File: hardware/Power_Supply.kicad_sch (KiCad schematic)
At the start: 50 parts, among them IC1 LM13700, IC2 LM13700, IC3 LM13700, J1 USB_B, SW2 POWER, U2 TL064, U6 TL064

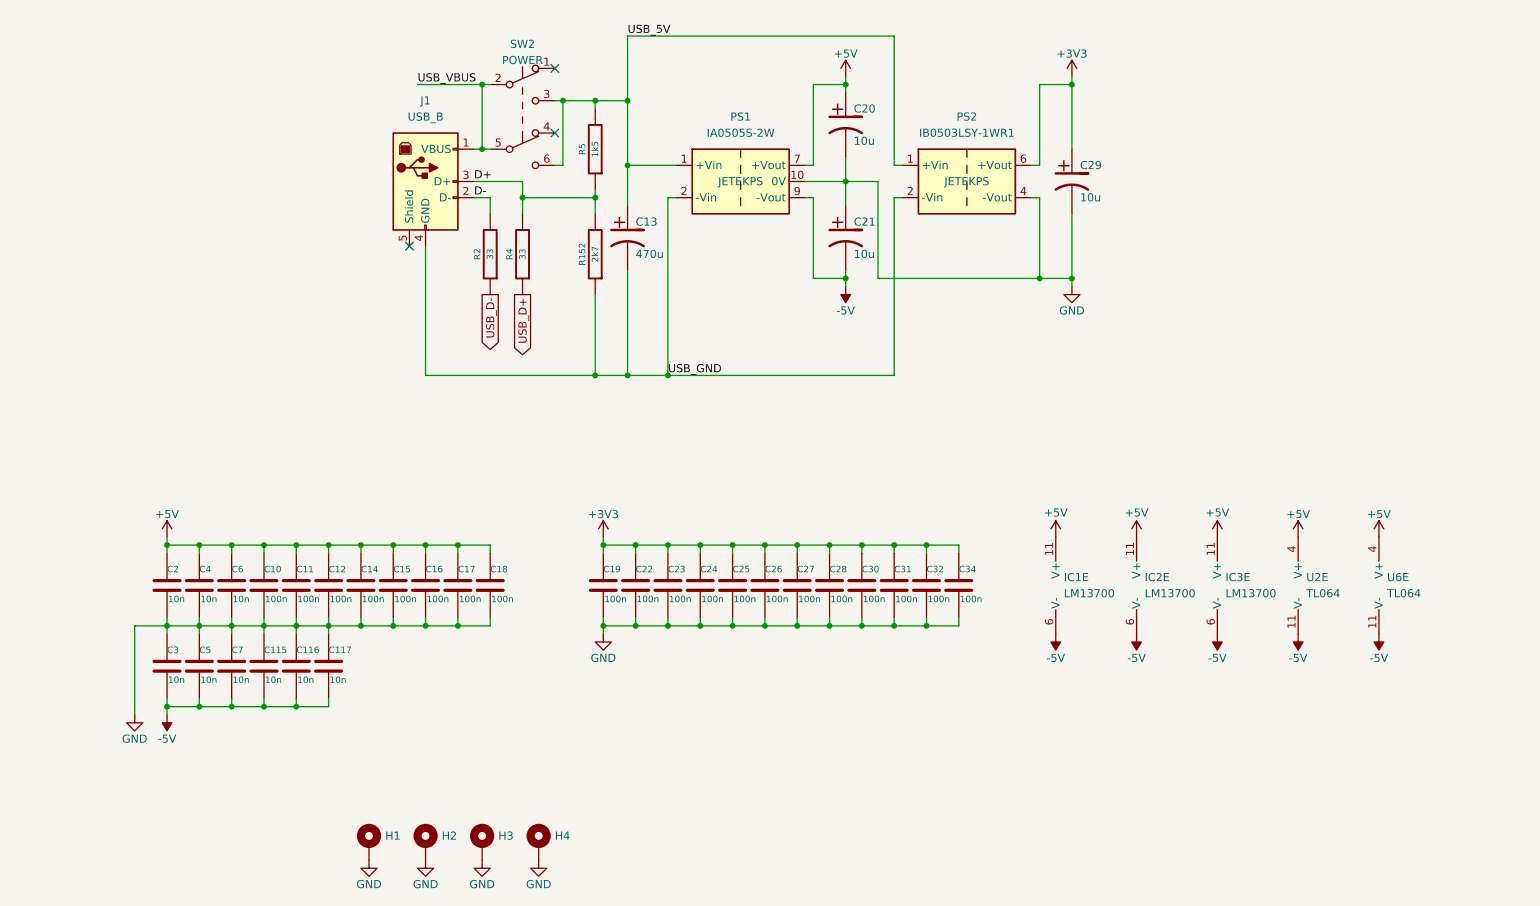
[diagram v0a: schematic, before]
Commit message: hardware: sch/pcb updates by Guimli
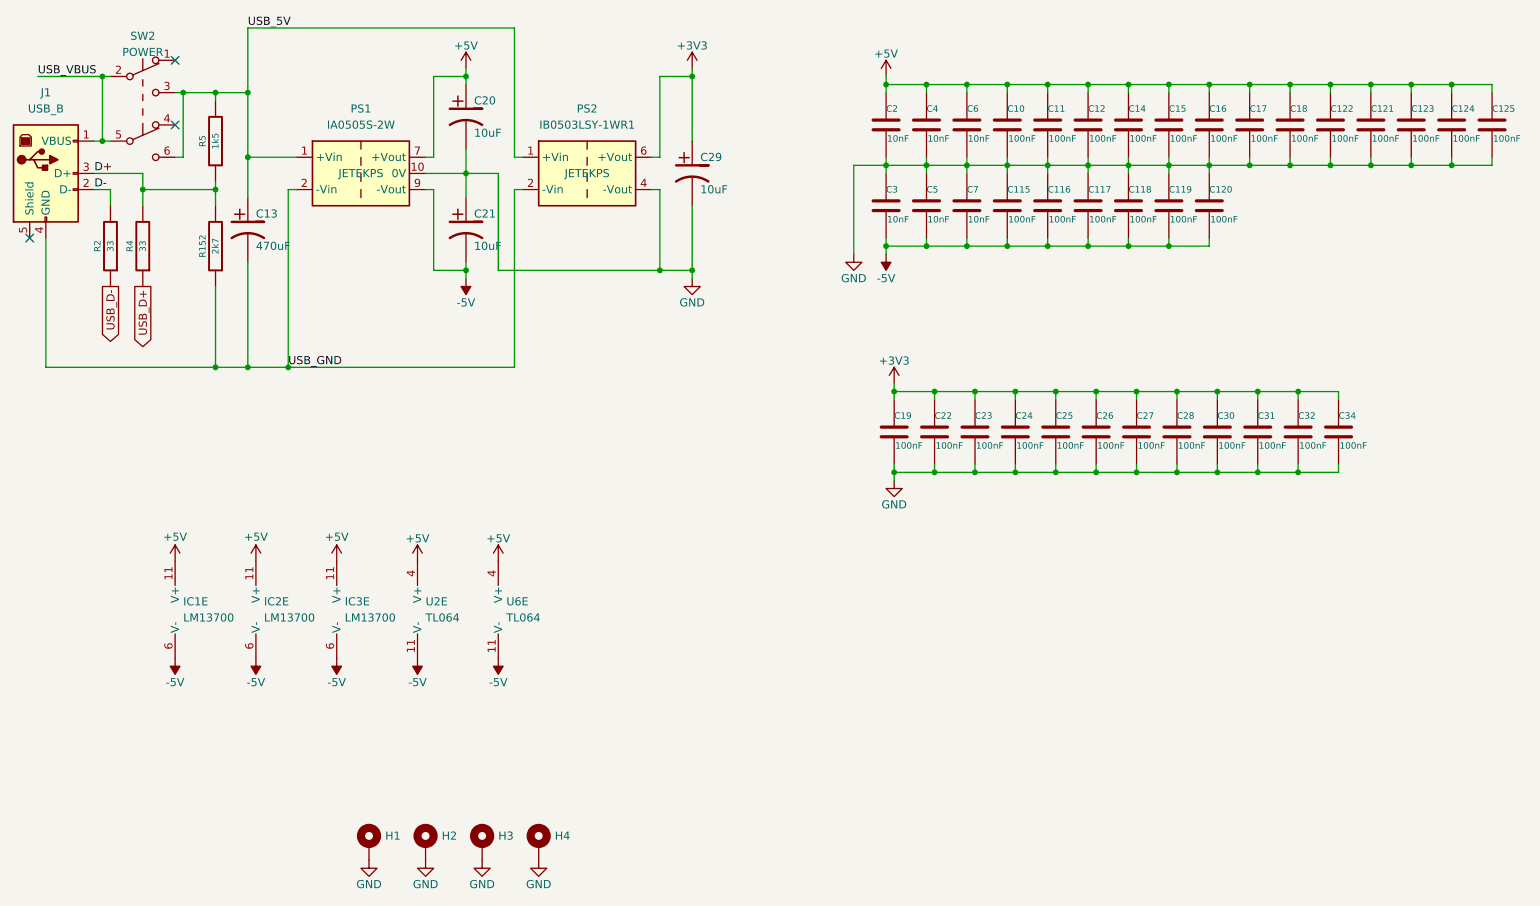
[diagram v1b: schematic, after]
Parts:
- added C118, C119, C120, C121, C122, C123, C124, C125: 100nF, Capacitor_SMD:C_0805_2012Metric, symbol Additional:C
- C10, C11, C12, C14, C15, C16, C17, C18, C19, C22, C23, C24, C25, C26, C27, C28, C30, C31, C32, C34: value 100n -> 100nF
- C115, C116, C117: value 10n -> 100nF; LCSC C1710 -> C28233
- C13: value 470u -> 470uF
- C2, C3, C4, C5, C6, C7: value 10n -> 10nF
- C20, C21, C29: value 10u -> 10uF
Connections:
- net +5V: now also C121.1, C122.1, C123.1, C124.1, C125.1
- net -5V: now also C118.2, C119.2, C120.2
- net GND: now also C118.1, C119.1, C120.1, C121.2, C122.2, C123.2, C124.2, C125.2
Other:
- moved on the sheet: C10, C11, C115, C116, C117, C12, C13, C14, C15, C16, C17, C18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
